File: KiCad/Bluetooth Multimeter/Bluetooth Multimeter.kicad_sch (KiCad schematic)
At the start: 33 parts, among them J1 V/Ohm, J2 Com, J3 mA, J4 A, J5 Parallel Prot, J6 3.3V, J7 GND, K1 Low Range, K2 Medium Range, K3 High Range, K4 UH Range (Ohm Only), K5 V/Ohm Switch, U1 ItsyBitsy_NRF52840_Big

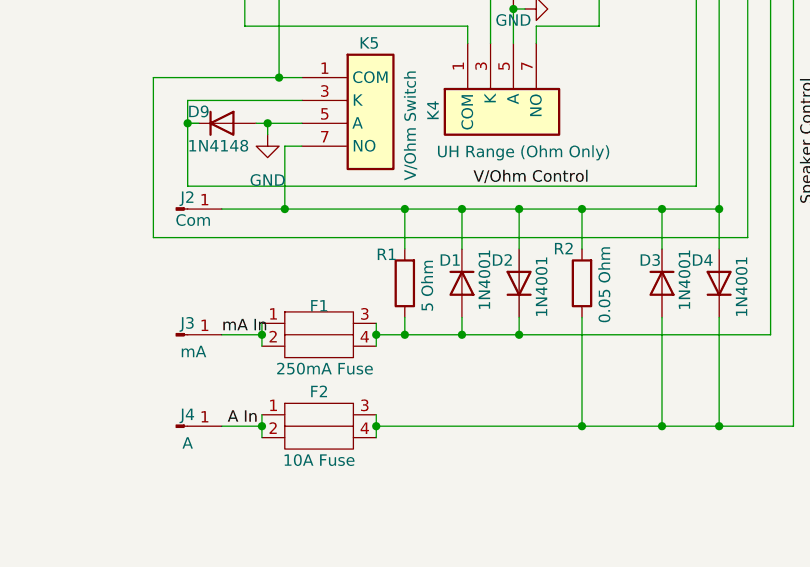
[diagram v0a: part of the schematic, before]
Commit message: finalized pcb rev 4 and sent to shop
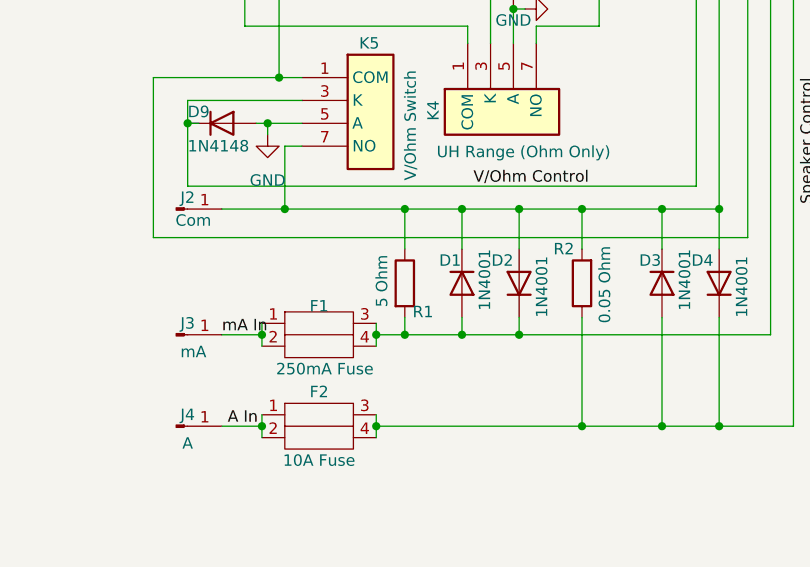
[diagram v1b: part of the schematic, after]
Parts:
- F1: footprint 502ProjectFootprints:LF124061_2 -> 502ProjectFootprints:LF124061_1
- F2: footprint 502ProjectFootprints:LF124041_3 -> 502ProjectFootprints:LF124041_4
- R1: footprint Resistor_THT:R_Axial_DIN0207_L6.3mm_D2.5mm_P10.16mm_Horizontal -> Resistor_THT:R_Axial_DIN0207_L6.3mm_D2.5mm_P2.54mm_Vertical
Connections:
- net Input Common: now also R1.1; no longer R1.2
- net mA ADC In: now also R1.2; no longer R1.1
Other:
- moved on the sheet: R1
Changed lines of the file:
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@@
     )
   )
-  (symbol (lib_id "Device:R") (at 107.95 161.29 180) (unit 1)
-    (in_bom yes) (on_board yes) (dnp no)
-    (property "Reference" "R1" (at 104.775 158.115 0)
+  (symbol (lib_id "Device:R") (at 107.95 161.29 0) (unit 1)
+    (in_bom yes) (on_board yes) (dnp no)
+    (property "Reference" "R1" (at 111.125 164.465 0)
       (effects (font (size 1.27 1.27)) (justify right))
     )
-    (property "Value" "5 Ohm" (at 110.49 164.465 90)
+    (property "Value" "5 Ohm" (at 105.41 158.115 90)
       (effects (font (size 1.27 1.27)) (justify right))
     )
-    (property "Footprint" "Resistor_THT:R_Axial_DIN0207_L6.3mm_D2.5mm_P10.16mm_Horizontal" (at 109.728 161.29 90)
+    (property "Footprint" "Resistor_THT:R_Axial_DIN0207_L6.3mm_D2.5mm_P2.54mm_Vertical" (at 106.172 161.29 90)
       (effects (font (size 1.27 1.27)) hide)
     )
@@
       (effects (font (size 1.27 1.27)))
     )
-    (property "Footprint" "502ProjectFootprints:LF124061_2" (at 92.075 161.925 0)
+    (property "Footprint" "502ProjectFootprints:LF124061_1" (at 92.075 161.925 0)
       (effects (font (size 1.27 1.27)) hide)
     )
@@
       (effects (font (size 1.27 1.27)))
     )
-    (property "Footprint" "502ProjectFootprints:LF124041_3" (at 92.075 172.085 0)
-      (effects (font (size 1.27 1.27)) hide)
-    )
+    (property "Footprint" "502ProjectFootprints:LF124041_4" (at 92.075 172.085 0)
+      (effects (font (size 1.27 1.27)) hide)
+    )
